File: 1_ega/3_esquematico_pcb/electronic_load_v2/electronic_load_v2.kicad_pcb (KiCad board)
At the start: 2 copper layers, 100 x 62.5 mm, 57 parts, among them J1 Encoder, J10 5V, J11 LOAD, J12 Memoria SD, J13 LCD, J15 VCC, J17 EGB_I2C, J2 RTC_I2C, J6 RPico PWR, Q1 IRF540N, Q3 BC327, Q4 BC327, SW1 BTN_MENU, SW2 BTN_STOP, SW3 SW_PWR, U1 TL072, U2 module_ina219, U3 LM7805_TO220, U4 TL072

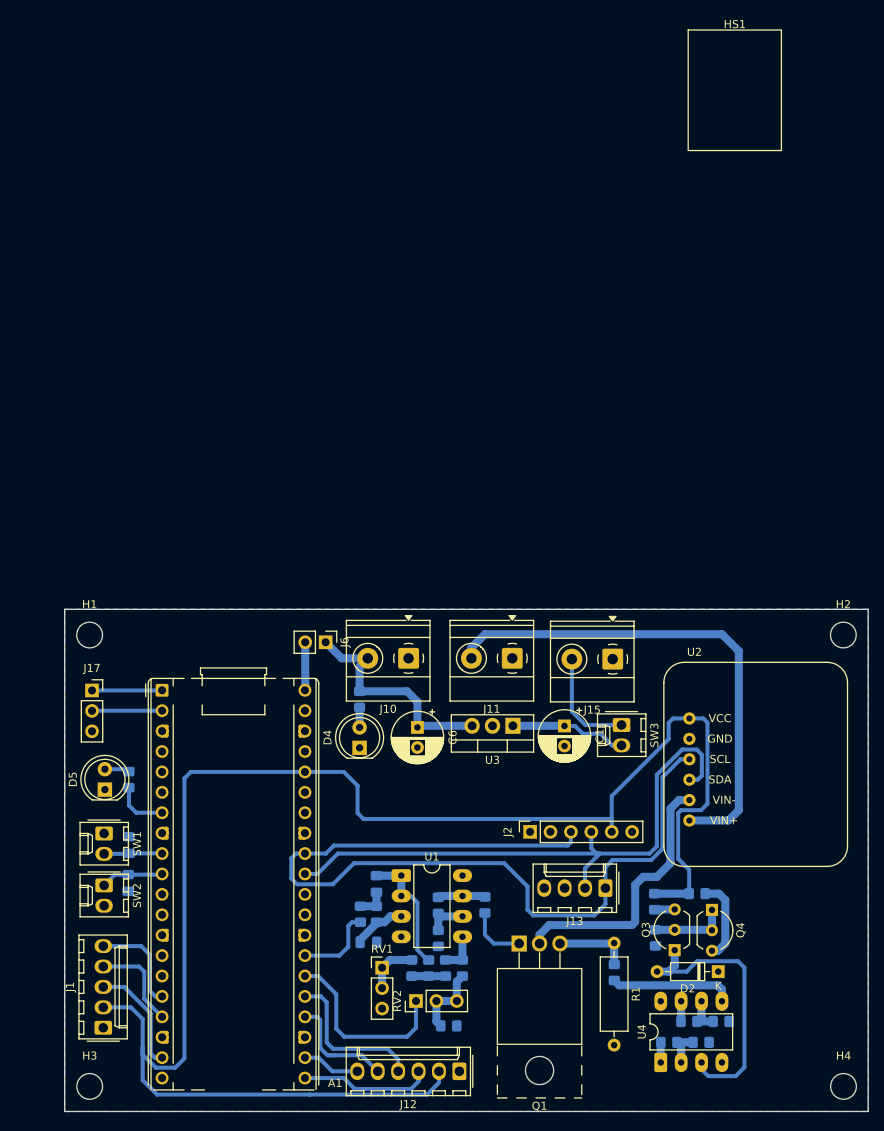
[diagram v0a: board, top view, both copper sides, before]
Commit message: chore: pcb v1 10x5 con R y C smd. INA modulo
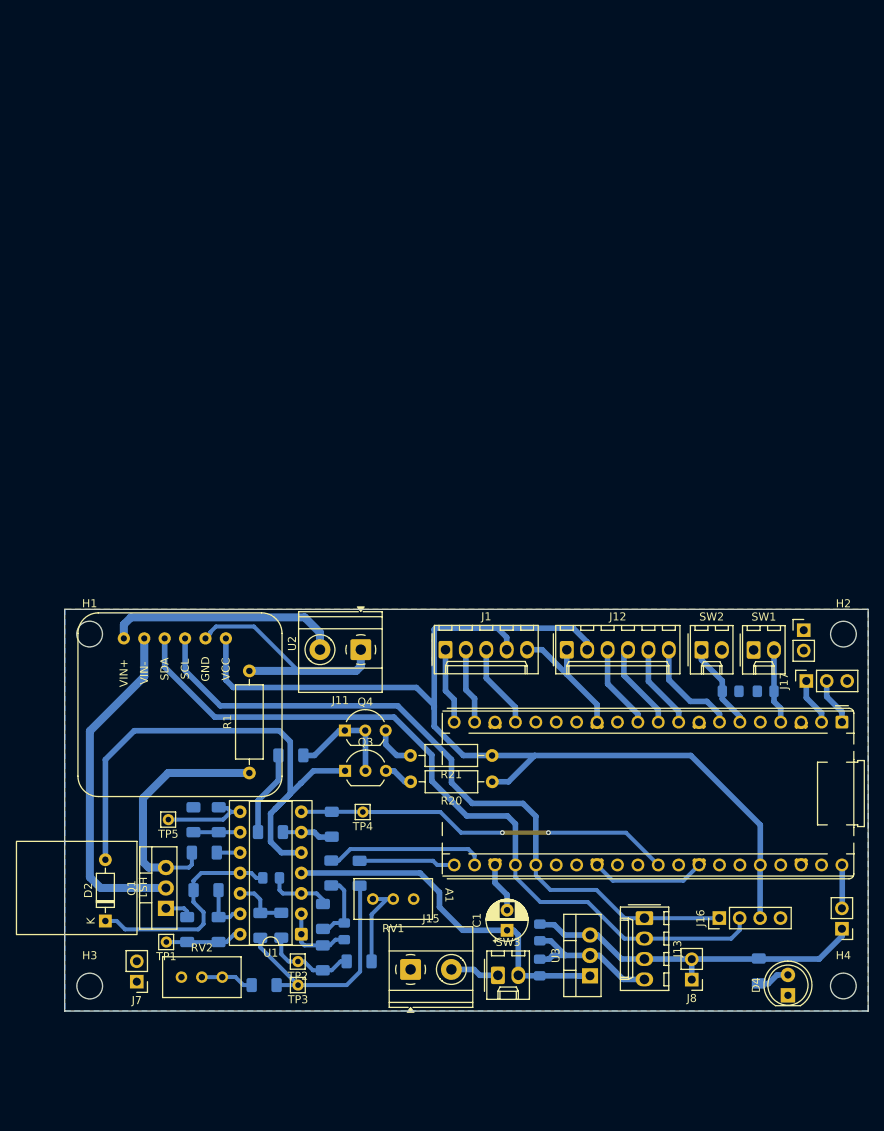
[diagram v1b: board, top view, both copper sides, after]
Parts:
- removed D5: LED_R, LED_THT:LED_D5.0mm
- removed J10: 5V, TerminalBlock_Phoenix:TerminalBlock_Phoenix_MKDS-1,5-2-5.08_1x02_P5.08mm_Horizontal
- removed J2: RTC_I2C, Connector_PinSocket_2.54mm:PinSocket_1x06_P2.54mm_Vertical
- removed R28: 150R, Resistor_SMD:R_0805_2012Metric_Pad1.20x1.40mm_HandSolder
- removed U4: TL072, Package_DIP:DIP-8_W7.62mm_LongPads
- added C7: 330nF, Capacitor_SMD:C_0805_2012Metric_Pad1.18x1.45mm_HandSolder, B.Cu at (79.1, 102.1)
- added J16: RTC, Connector_PinHeader_2.54mm:PinHeader_1x04_P2.54mm_Vertical, F.Cu at (101.5, 95.9)
- added J3: GND, Connector_PinHeader_2.54mm:PinHeader_1x02_P2.54mm_Vertical, F.Cu at (112.0, 60.1)
- added J7: GND, Connector_PinHeader_2.54mm:PinHeader_1x02_P2.54mm_Vertical, F.Cu at (29.0, 103.8)
- added J8: 5V, Connector_PinHeader_2.54mm:PinHeader_1x02_P2.54mm_Vertical, F.Cu at (98.0, 103.6)
- added R30: 3.3k, Resistor_SMD:R_1206_3216Metric_Pad1.30x1.75mm_HandSolder, B.Cu at (44.8, 104.3)
- added TP1: MOS_GATE, Connector_Pin:Pin_D0.7mm_L6.5mm_W1.8mm_FlatFork, F.Cu at (32.6, 98.9)
- added TP2: MOS_SK, Connector_Pin:Pin_D0.7mm_L6.5mm_W1.8mm_FlatFork, F.Cu at (49.0, 101.3)
- added TP3: MOS_OFFSET, Connector_Pin:Pin_D0.7mm_L6.5mm_W1.8mm_FlatFork, F.Cu at (49.0, 104.3)
- added TP4: T_DIODE, Connector_Pin:Pin_D0.7mm_L6.5mm_W1.8mm_FlatFork, F.Cu at (57.1, 82.7)
- added TP5: Isense, Connector_Pin:Pin_D0.7mm_L6.5mm_W1.8mm_FlatFork, F.Cu at (32.9, 83.7)
- C1: value 10uF -> 100uF; footprint Capacitor_THT:CP_Radial_D6.3mm_P2.50mm -> Capacitor_THT:CP_Radial_D5.0mm_P2.50mm
- C6: value 10uF -> 100nF; footprint Capacitor_THT:CP_Radial_D6.3mm_P2.50mm -> Capacitor_SMD:C_0805_2012Metric_Pad1.18x1.45mm_HandSolder; moved to B.Cu
- Q1: footprint Package_TO_SOT_THT:TO-220F-3_Horizontal_TabUp -> Package_TO_SOT_THT:TO-220-3_Vertical
- R11, R12, R14, R15, R16, R17, R18, R19, R22, R23, R24, R25, R26, R27, R29, R6, R7: footprint Resistor_SMD:R_0805_2012Metric_Pad1.20x1.40mm_HandSolder -> Resistor_SMD:R_1206_3216Metric_Pad1.30x1.75mm_HandSolder
- R20, R21: footprint Resistor_SMD:R_0805_2012Metric_Pad1.20x1.40mm_HandSolder -> Resistor_THT:R_Axial_DIN0207_L6.3mm_D2.5mm_P10.16mm_Horizontal; moved to F.Cu
- RV1, RV2: footprint Connector_PinHeader_2.54mm:PinHeader_1x03_P2.54mm_Vertical -> Potentiometer_THT:Potentiometer_Bourns_3296W_Vertical
- U1: value TL072 -> LM324; footprint Package_DIP:DIP-8_W7.62mm_LongPads -> Package_DIP:DIP-14_W7.62mm_Socket
- moved HS1 130.2 mm to (29.2, 92.2), turned to -90 degrees
- moved J17 88.9 mm to (112.3, 66.4), turned to 90 degrees
- moved SW1 84.0 mm to (105.7, 62.6), turned to 0 degrees
- moved C3 81.5 mm to (107.2, 67.7), turned to 0 degrees
- moved SW2 79.9 mm to (99.2, 62.5), turned to 0 degrees
- moved C4 78.7 mm to (102.9, 67.7), turned to 180 degrees
- moved D2 76.5 mm to (25.1, 96.3), turned to 90 degrees
- moved U2 73.9 mm to (27.4, 61.1), turned to -90 degrees
- moved J6 73.5 mm to (116.7, 97.3), turned to 180 degrees
- moved R26 70.3 mm to (36.0, 83.7), turned to -90 degrees
- moved R29 63.7 mm to (39.2, 83.7), turned to 90 degrees
- moved J1 63.5 mm to (67.4, 62.5), turned to 0 degrees
- moved D4 61.6 mm to (110.0, 105.5)
- moved R27 60.1 mm to (106.4, 102.5)
- moved R14 59.6 mm to (45.6, 85.2), turned to 180 degrees
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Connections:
- A1 pad 10: BTN_STOP -> SPI0_TX
- A1 pad 11: TX_EGB -> SPI0_CS
- A1 pad 12: RX_EGB -> unconnected-(A1-GPIO9-Pad12)
- A1 pad 16: ENC_CLK -> unconnected-(A1-GPIO12-Pad16)
- A1 pad 17: ENC_DT -> ENC_SW
- A1 pad 19: ENC_SW -> ENC_DT
- A1 pad 20: unconnected-(A1-GPIO15-Pad20) -> ENC_CLK
- A1 pad 21: SPI0_RX -> MOS_EN
- A1 pad 22: SPI0_CS -> MOS_PWM
- A1 pad 24: SPI0_CLK -> I2C_SDA
- A1 pad 25: SPI0_TX -> I2C_SCL
- A1 pad 26: MOS_EN -> unconnected-(A1-GPIO20-Pad26)
- A1 pad 27: MOS_PWM -> unconnected-(A1-GPIO21-Pad27)
- A1 pad 31: I2C_SDA -> TEMP_DIODE
- A1 pad 32: I2C_SCL -> unconnected-(A1-GPIO27_ADC1-Pad32)
- A1 pad 33: unconnected-(A1-AGND-Pad33) -> GND
- A1 pad 34: TEMP_DIODE -> unconnected-(A1-GPIO28_ADC2-Pad34)
- A1 pad 4: unconnected-(A1-GPIO2-Pad4) -> BTN_MENU
- A1 pad 6: unconnected-(A1-GPIO4-Pad6) -> BTN_STOP
- A1 pad 7: LED_ACTIVE -> SPI0_RX
- A1 pad 9: BTN_MENU -> SPI0_CLK
- C6 pad 1: +5V -> GND
- C6 pad 2: GND -> +5V
- J1 pad 1: GND -> ENC_CLK
- J1 pad 2: +3V3 -> ENC_DT
- J1 pad 4: ENC_DT -> +3V3
- J1 pad 5: ENC_CLK -> GND
- J12 pad 3: SPI0_RX -> SPI0_CS
- J12 pad 6: SPI0_CS -> SPI0_RX
- J17 pad 1: EGB_TX_SDA -> EGB_RX_SCL
- J17 pad 2: EGB_RX_SCL -> EGB_TX_SDA
- R14 pad 1: Net-(U4A--) -> Net-(U1B--)
- R15 pad 1: Net-(U4A--) -> Net-(U1B--)
- R16 pad 1: GND -> MOS_OFFSET
- R16 pad 2: MOS_OFFSET -> MOS_EN
- R17 pad 2: Net-(U1B-+) -> Net-(U1D-+)
- R22 pad 2: Net-(U1B-+) -> Net-(U1D-+)
- R23 pad 1: Net-(U1B--) -> Net-(U1D--)
- R24 pad 2: Net-(U1B--) -> Net-(U1D--)
- R25 pad 2: Net-(U4B-+) -> Net-(U1C-+)
- R26 pad 2: Net-(U4B--) -> Net-(U1C--)
- R29 pad 1: Net-(U4B--) -> Net-(U1C--)
- RV2 pad 1: MOS_EN -> Net-(R30-Pad1)
- RV2 pad 2: MOS_OFFSET -> Net-(R30-Pad1)
- RV2 pad 3: MOS_OFFSET -> GND
- U1 pad 4: GND -> VCC
- U1 pad 5: Net-(U1B-+) -> Net-(D2-A)
- U1 pad 7: MOS_GATE -> TEMP_DIODE
- U1 pad 8: VCC -> Io_sens
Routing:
- net GND: track 0.00 -> 125.2 mm
- net +3V3: track 203.7 -> 133.0 mm
- net TEMP_DIODE: track 2.51 -> 47.2 mm, vias 0 -> 2
- net LOAD+: track 62.7 -> 29.4 mm
- net VCC: track 14.9 -> 47.0 mm
- net Net-(D2-A): track 35.6 -> 66.4 mm
- net I2C_SDA: track 73.7 -> 96.9 mm
- net I2C_SCL: track 110.7 -> 89.3 mm
- net I_sens: track 9.43 -> 30.5 mm
- net MOS_OFFSET: track 9.25 -> 29.6 mm
- net +5V: track 28.4 -> 44.1 mm
- net Net-(U4B-+): track 15.3 -> 0.00 mm
- net MOS_EN: track 23.3 -> 12.0 mm
- net MOS_PWM: track 10.1 -> 19.9 mm
- net MOS_DRAIN: track 33.4 -> 42.5 mm
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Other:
- board size 100 x 62.5 mm -> 100 x 50 mm
